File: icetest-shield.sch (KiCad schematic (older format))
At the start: 10 parts

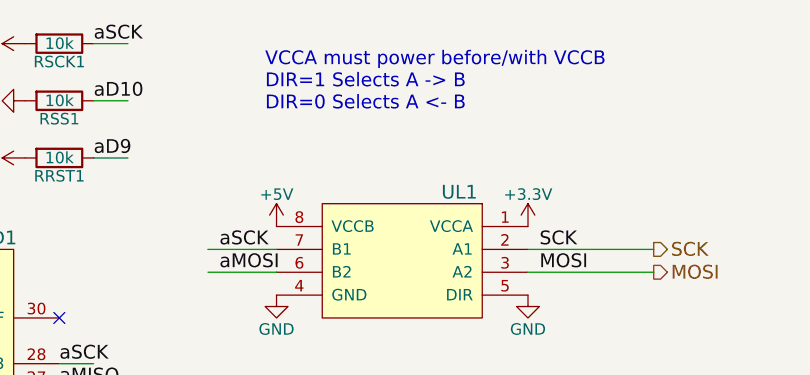
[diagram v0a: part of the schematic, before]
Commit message: more layout
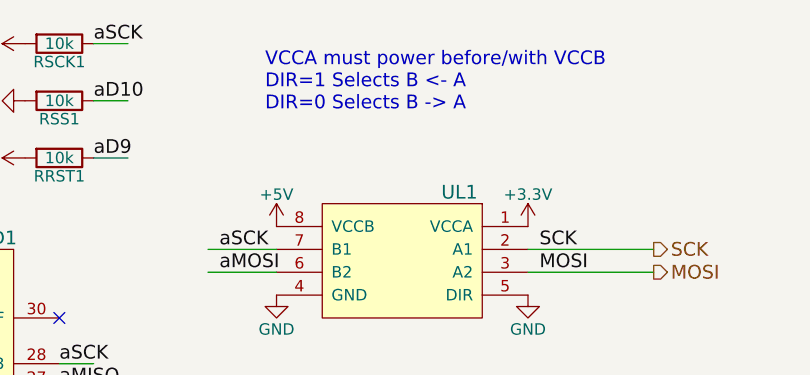
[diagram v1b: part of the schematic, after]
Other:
- note added: "VCCA must power before/with VCCB\nDIR=1 Selects B <- A\nDIR=0 Selects B -> A"
- note removed: "VCCA must power before/with VCCB\nDIR=1 Selects A -> B\nDIR=0 Selects A <- B"
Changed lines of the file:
@@
 $EndComp
 $Comp
-L GND #PWR049
+L GND #PWR050
 U 1 1 578B7F2F
 P 4100 3400
-F 0 "#PWR049" H 4100 3150 50  0001 C CNN
+F 0 "#PWR050" H 4100 3150 50  0001 C CNN
 F 1 "GND" H 4100 3250 50  0000 C CNN
 F 2 "" H 4100 3400 50  0000 C CNN
@@
 $EndComp
 $Comp
-L +5V #PWR050
+L +5V #PWR051
 U 1 1 578B7F35
 P 3900 3050
-F 0 "#PWR050" H 3900 2900 50  0001 C CNN
+F 0 "#PWR051" H 3900 2900 50  0001 C CNN
 F 1 "+5V" H 3900 3190 50  0000 C CNN
 F 2 "" H 3900 3050 50  0000 C CNN
@@
 NoConn ~ 5950 2750
 $Comp
-L +3.3V #PWR051
+L +3.3V #PWR052
 U 1 1 578B7F8A
 P 8000 2350
-F 0 "#PWR051" H 8000 2200 50  0001 C CNN
+F 0 "#PWR052" H 8000 2200 50  0001 C CNN
 F 1 "+3.3V" H 8000 2490 50  0000 C CNN
 F 2 "" H 8000 2350 50  0000 C CNN
@@
 $EndComp
 $Comp
-L +5V #PWR052
+L +5V #PWR053
 U 1 1 578B7F90
 P 6900 2350
-F 0 "#PWR052" H 6900 2200 50  0001 C CNN
+F 0 "#PWR053" H 6900 2200 50  0001 C CNN
 F 1 "+5V" H 6900 2490 50  0000 C CNN
 F 2 "" H 6900 2350 50  0000 C CNN
@@
 ICE_CDONE
 $Comp
-L GND #PWR053
+L GND #PWR054
 U 1 1 5793C5E6
 P 5100 4700
-F 0 "#PWR053" H 5100 4450 50  0001 C CNN
+F 0 "#PWR054" H 5100 4450 50  0001 C CNN
 F 1 "GND" H 5100 4550 50  0000 C CNN
 F 2 "" H 5100 4700 50  0000 C CNN
@@
 $EndComp
 $Comp
-L GND #PWR054
+L GND #PWR055
 U 1 1 57F9B00B
 P 6900 2650
-F 0 "#PWR054" H 6900 2400 50  0001 C CNN
+F 0 "#PWR055" H 6900 2400 50  0001 C CNN
 F 1 "GND" H 6900 2500 50  0000 C CNN
 F 2 "" H 6900 2650 50  0000 C CNN
@@
 $EndComp
 Text Notes 6850 1850 0    60   ~ 0
-VCCA must power before/with VCCB\nDIR=1 Selects A -> B\nDIR=0 Selects A <- B
-$Comp
-L GND #PWR055
+VCCA must power before/with VCCB\nDIR=1 Selects B <- A\nDIR=0 Selects B -> A
+$Comp
+L GND #PWR056
 U 1 1 57F9C120
 P 8000 2650
-F 0 "#PWR055" H 8000 2400 50  0001 C CNN
+F 0 "#PWR056" H 8000 2400 50  0001 C CNN
 F 1 "GND" H 8000 2500 50  0000 C CNN
 F 2 "" H 8000 2650 50  0000 C CNN
@@
 $EndComp
 $Comp
-L +3.3V #PWR056
+L +3.3V #PWR057
 U 1 1 57F9C181
 P 8000 3200
-F 0 "#PWR056" H 8000 3050 50  0001 C CNN
+F 0 "#PWR057" H 8000 3050 50  0001 C CNN
 F 1 "+3.3V" H 8000 3340 50  0000 C CNN
 F 2 "" H 8000 3200 50  0000 C CNN
@@
 $EndComp
 $Comp
-L +5V #PWR057
+L +5V #PWR058
 U 1 1 57F9C187
 P 6900 3200
-F 0 "#PWR057" H 6900 3050 50  0001 C CNN
+F 0 "#PWR058" H 6900 3050 50  0001 C CNN
 F 1 "+5V" H 6900 3340 50  0000 C CNN
 F 2 "" H 6900 3200 50  0000 C CNN
@@
 $EndComp
 $Comp
-L GND #PWR058
+L GND #PWR059
 U 1 1 57F9C193
 P 6900 3500
-F 0 "#PWR058" H 6900 3250 50  0001 C CNN
+F 0 "#PWR059" H 6900 3250 50  0001 C CNN
 F 1 "GND" H 6900 3350 50  0000 C CNN
 F 2 "" H 6900 3500 50  0000 C CNN
@@
 $EndComp
 $Comp
-L GND #PWR059
+L GND #PWR060
 U 1 1 57F9C199
 P 8000 3500
-F 0 "#PWR059" H 8000 3250 50  0001 C CNN
+F 0 "#PWR060" H 8000 3250 50  0001 C CNN
 F 1 "GND" H 8000 3350 50  0000 C CNN
 F 2 "" H 8000 3500 50  0000 C CNN
@@
 $EndComp
 $Comp
-L +3.3V #PWR060
+L +3.3V #PWR061
 U 1 1 57F9C239
 P 8000 4000
-F 0 "#PWR060" H 8000 3850 50  0001 C CNN
+F 0 "#PWR061" H 8000 3850 50  0001 C CNN
 F 1 "+3.3V" H 8000 4140 50  0000 C CNN
 F 2 "" H 8000 4000 50  0000 C CNN
@@
 $EndComp
 $Comp
-L +5V #PWR061
+L +5V #PWR062
 U 1 1 57F9C23F
 P 6900 4000
-F 0 "#PWR061" H 6900 3850 50  0001 C CNN
+F 0 "#PWR062" H 6900 3850 50  0001 C CNN
 F 1 "+5V" H 6900 4140 50  0000 C CNN
 F 2 "" H 6900 4000 50  0000 C CNN
@@
 $EndComp
 $Comp
-L GND #PWR062
+L GND #PWR063
 U 1 1 57F9C24B
 P 6900 4300
-F 0 "#PWR062" H 6900 4050 50  0001 C CNN
+F 0 "#PWR063" H 6900 4050 50  0001 C CNN
 F 1 "GND" H 6900 4150 50  0000 C CNN
 F 2 "" H 6900 4300 50  0000 C CNN
@@
 $EndComp
 $Comp
-L +3.3V #PWR063
+L +3.3V #PWR064
 U 1 1 57F9C281
 P 8000 4750
-F 0 "#PWR063" H 8000 4600 50  0001 C CNN
+F 0 "#PWR064" H 8000 4600 50  0001 C CNN
 F 1 "+3.3V" H 8000 4890 50  0000 C CNN
 F 2 "" H 8000 4750 50  0000 C CNN
@@
 $EndComp
 $Comp
-L +5V #PWR064
+L +5V #PWR065
 U 1 1 57F9C287
 P 6900 4750
-F 0 "#PWR064" H 6900 4600 50  0001 C CNN
+F 0 "#PWR065" H 6900 4600 50  0001 C CNN
 F 1 "+5V" H 6900 4890 50  0000 C CNN
 F 2 "" H 6900 4750 50  0000 C CNN
@@
 $EndComp
 $Comp
-L GND #PWR065
+L GND #PWR066
 U 1 1 57F9C293
 P 6900 5050
-F 0 "#PWR065" H 6900 4800 50  0001 C CNN
+F 0 "#PWR066" H 6900 4800 50  0001 C CNN
 F 1 "GND" H 6900 4900 50  0000 C CNN
 F 2 "" H 6900 5050 50  0000 C CNN
@@
 $EndComp
 $Comp
-L GND #PWR066
+L GND #PWR067
 U 1 1 57F9C299
 P 8000 5650
-F 0 "#PWR066" H 8000 5400 50  0001 C CNN
+F 0 "#PWR067" H 8000 5400 50  0001 C CNN
 F 1 "GND" H 8000 5500 50  0000 C CNN
 F 2 "" H 8000 5650 50  0000 C CNN
@@
 $EndComp
 $Comp
-L GND #PWR067
+L GND #PWR068
 U 1 1 57FA17AB
 P 5800 1800
-F 0 "#PWR067" H 5800 1550 50  0001 C CNN
+F 0 "#PWR068" H 5800 1550 50  0001 C CNN
 F 1 "GND" H 5800 1650 50  0000 C CNN
 F 2 "" H 5800 1800 50  0000 C CNN
@@
 DD
 $Comp
-L +5V #PWR068
+L +5V #PWR069
 U 1 1 57FC7EF2
 P 5800 1550
-F 0 "#PWR068" H 5800 1400 50  0001 C CNN
+F 0 "#PWR069" H 5800 1400 50  0001 C CNN
 F 1 "+5V" H 5800 1690 50  0000 C CNN
 F 2 "" H 5800 1550 50  0000 C CNN
@@
 $EndComp
 $Comp
-L +5V #PWR069
+L +5V #PWR070
 U 1 1 57FC7F18
 P 5800 2050
-F 0 "#PWR069" H 5800 1900 50  0001 C CNN
+F 0 "#PWR070" H 5800 1900 50  0001 C CNN
 F 1 "+5V" H 5800 2190 50  0000 C CNN
 F 2 "" H 5800 2050 50  0000 C CNN
@@
 	8400 4300 8550 4300
 $Comp
-L +3.3V #PWR070
+L +3.3V #PWR071
 U 1 1 57FAE2AA
 P 8550 4300
-F 0 "#PWR070" H 8550 4150 50  0001 C CNN
+F 0 "#PWR071" H 8550 4150 50  0001 C CNN
 F 1 "+3.3V" H 8550 4440 50  0000 C CNN
 F 2 "" H 8550 4300 50  0000 C CNN
